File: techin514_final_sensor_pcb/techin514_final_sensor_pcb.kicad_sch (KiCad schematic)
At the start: 14 parts, among them J1 28BYJ-48 Stepper Motor, SW1 CK_KMS2xxGP, U1 ESP32-C3-DevKitM-1, U2 ESP32-C3-DevKitM-1, U3 ADXL343, U4 ULN2003, U5 TPS79301-EP

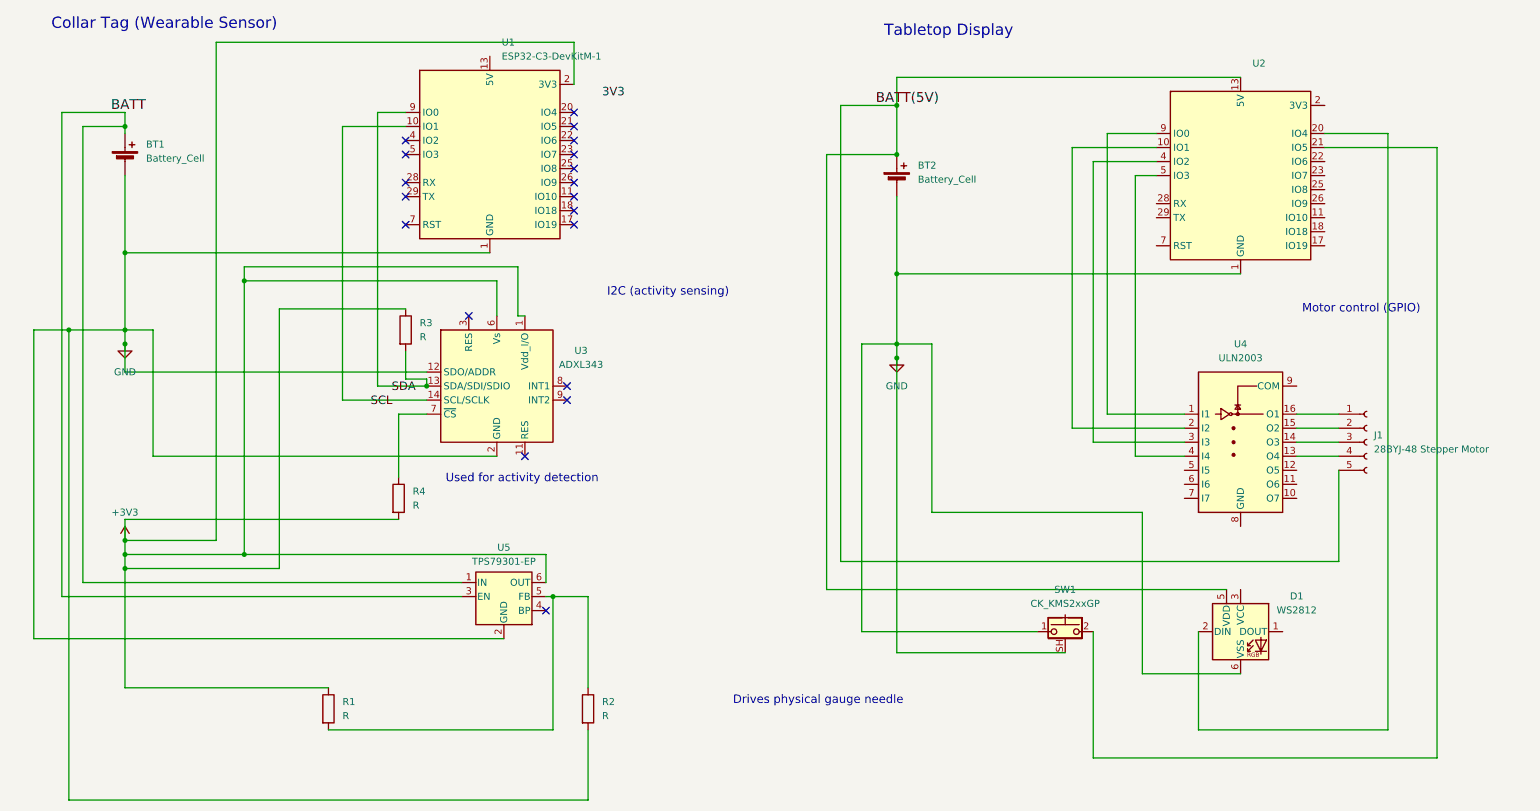
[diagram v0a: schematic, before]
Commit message: update pcb
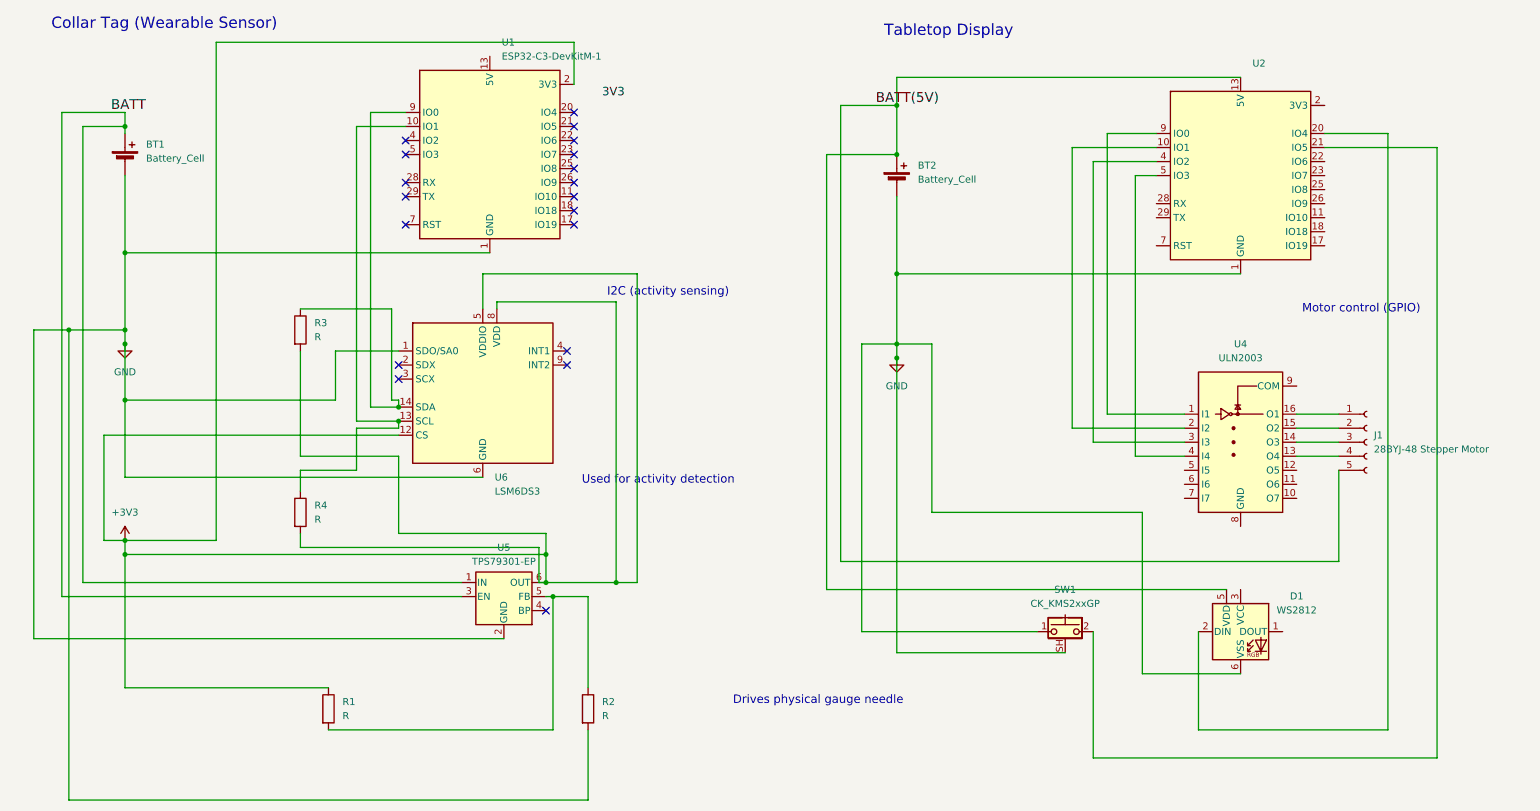
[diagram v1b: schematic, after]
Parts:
- removed U3: ADXL343, Package_LGA:LGA-14_3x5mm_P0.8mm_LayoutBorder1x6y, symbol Sensor_Motion:ADXL343
- added U6: LSM6DS3, Package_LGA:LGA-14_3x2.5mm_P0.5mm_LayoutBorder3x4y, symbol Sensor_Motion:LSM6DS3
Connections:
- net +3V3: now also R3.2, U6.12 (CS), U6.5 (VDDIO), U6.8 (VDD); no longer R3.1
- net GND: now also U6.1 (SDO/SA0), U6.6 (GND), U6.7 (GND)
- net at U1.9 (IO0): now also R3.1, U6.14 (SDA); no longer R3.2
- net at U1.10 (IO1): now also R4.1, U6.13 (SCL)
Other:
- moved on the sheet: R3, R4

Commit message: updated schematic and PCB
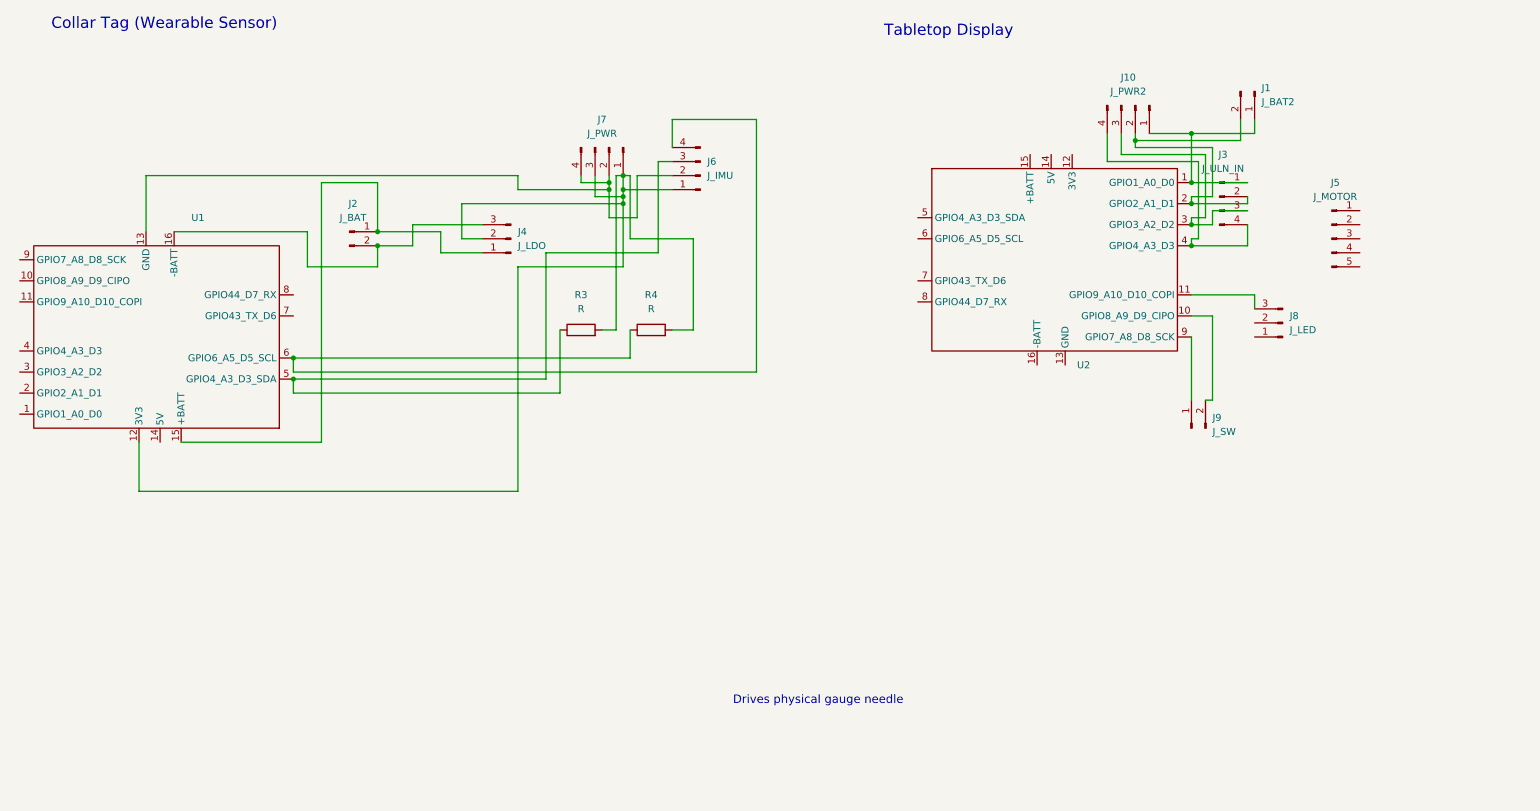
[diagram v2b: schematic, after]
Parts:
- removed BT1: Battery_Cell, Battery:BatteryHolder_Bulgin_BX0034_1xAAA, symbol Device:Battery_Cell
- removed BT2: Battery_Cell, Connector_PinHeader_1.00mm:PinHeader_1x02_P1.00mm_Vertical, symbol Device:Battery_Cell
- removed D1: WS2812, LED_SMD:LED_WS2812_PLCC6_5.0x5.0mm_P1.6mm, symbol LED:WS2812
- removed J1: 28BYJ-48 Stepper Motor, Connector_PinHeader_1.00mm:PinHeader_1x05_P1.00mm_Vertical, symbol Connector:Conn_01x05_Socket
- removed R1, R2: R, Resistor_SMD:R_0603_1608Metric, symbol Device:R
- removed SW1: CK_KMS2xxGP, Button_Switch_SMD:SW_Push_1P1T-SH_NO_CK_KMR2xxG, symbol Switch:CK_KMS2xxGP
- removed U1, U2: ESP32-C3-DevKitM-1, RF_Module:ESP32-C3-DevKitM-1, symbol RF_Module:ESP32-C3-DevKitM-1
- removed U4: ULN2003, Package_DIP:DIP-16_W7.62mm, symbol Transistor_Array:ULN2003
- removed U5: TPS79301-EP, Package_SON:SON-8-1EP_3x2mm_P0.5mm_EP1.4x1.6mm, symbol Regulator_Linear:TPS79301-EP
- removed U6: LSM6DS3, Package_LGA:LGA-14_3x2.5mm_P0.5mm_LayoutBorder3x4y, symbol Sensor_Motion:LSM6DS3
- added J1: J_BAT2, Connector_PinHeader_2.54mm:PinHeader_1x02_P2.54mm_Vertical, symbol Connector:Conn_01x02_Pin
- added J10: J_PWR2, Connector_PinHeader_2.54mm:PinHeader_1x04_P2.54mm_Vertical, symbol Connector:Conn_01x04_Pin
- added J2: J_BAT, Connector_PinHeader_2.54mm:PinHeader_1x02_P2.54mm_Vertical, symbol Connector:Conn_01x02_Pin
- added J3: J_ULN_IN, Connector_PinHeader_2.54mm:PinHeader_1x04_P2.54mm_Vertical, symbol Connector:Conn_01x04_Pin
- added J4: J_LDO, Connector_PinHeader_2.54mm:PinHeader_1x02_P2.54mm_Vertical, symbol Connector:Conn_01x03_Pin
- added J5: J_MOTOR, Connector_PinHeader_2.54mm:PinHeader_1x05_P2.54mm_Vertical, symbol Connector:Conn_01x05_Pin
- added J6: J_IMU, Connector_PinHeader_2.54mm:PinHeader_1x04_P2.54mm_Vertical, symbol Connector:Conn_01x04_Pin
- added J7: J_PWR, Connector_PinHeader_2.54mm:PinHeader_1x02_P2.54mm_Vertical, symbol Connector:Conn_01x04_Pin
- added J8: J_LED, Connector_PinHeader_2.54mm:PinHeader_1x03_P2.54mm_Vertical, symbol Connector:Conn_01x03_Pin
- added J9: J_SW, Connector_PinHeader_2.54mm:PinHeader_1x02_P2.54mm_Vertical, symbol Connector:Conn_01x02_Pin
- added U1, U2: ~, ESP32footprint:XIAO_ESP32, symbol GIX_ESP32:XIAO_ESP32
- R3, R4: footprint Resistor_SMD:R_0603_1608Metric -> Resistor_THT:R_Axial_DIN0207_L6.3mm_D2.5mm_P7.62mm_Horizontal
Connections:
- net at R4.1: now also J6.4 (SCL), U1.6 (GPIO6_A5_D5_SCL)
- net at R3.1: now also J6.3 (SDA), U1.5 (GPIO4_A3_D3_SDA)
- net +3V3: no longer names the net of R3.2, R4.2
- net +3V3: now also J4.2 (3V3), J6.1 (3V3), J7.1 (3V3), J7.3 (3V3), U1.12 (3V3)
- new net: J1.1 (VBAT_5V), J10.1 (3V3), J3.1 (MOTOR_IN1), U2.1 (GPIO1_A0_D0)
- new net: J1.2 (GND), J10.2 (GND), J3.2 (MOTOR_IN2), U2.2 (GPIO2_A1_D1)
- new net: J10.3 (3V3), J3.3 (MOTOR_IN3), U2.3 (GPIO3_A2_D2)
- new net: J10.4 (GND), J3.4 (Pin_4), U2.4 (GPIO4_A3_D3)
- new net: J8.3 (LED_DIN), U2.11 (GPIO9_A10_D10_COPI)
- new net: J6.2 (GND), J7.2 (GND), J7.4 (GND), U1.13 (GND)
- new net: J9.2 (Pin_2), U2.10 (GPIO8_A9_D9_CIPO)
- new net: J9.1 (BTN), U2.9 (GPIO7_A8_D8_SCK)
- new net: J2.1 (VBAT), J4.1 (VBAT), U1.15 (+BATT)
- new net: J2.2 (GND), J4.3 (GND), U1.16 (-BATT)
- no-connect marks 19 -> 0
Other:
- note removed: "I2C (activity sensing)"
- note removed: "Motor control (GPIO)"
- note removed: "Used for activity detection"
